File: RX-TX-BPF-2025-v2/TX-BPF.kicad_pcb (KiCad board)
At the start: 11 copper layers, 60.6 x 26.8 mm, 21 parts

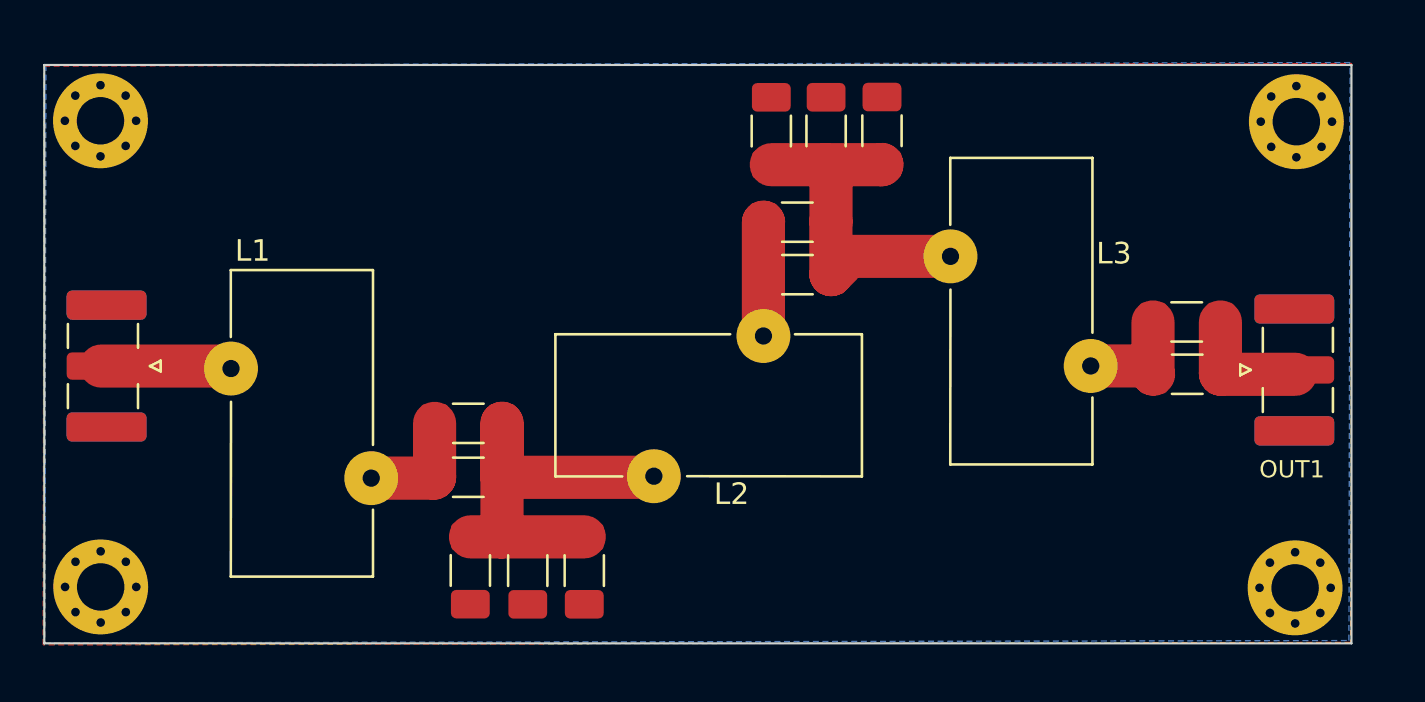
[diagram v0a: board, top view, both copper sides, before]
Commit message: A new start...
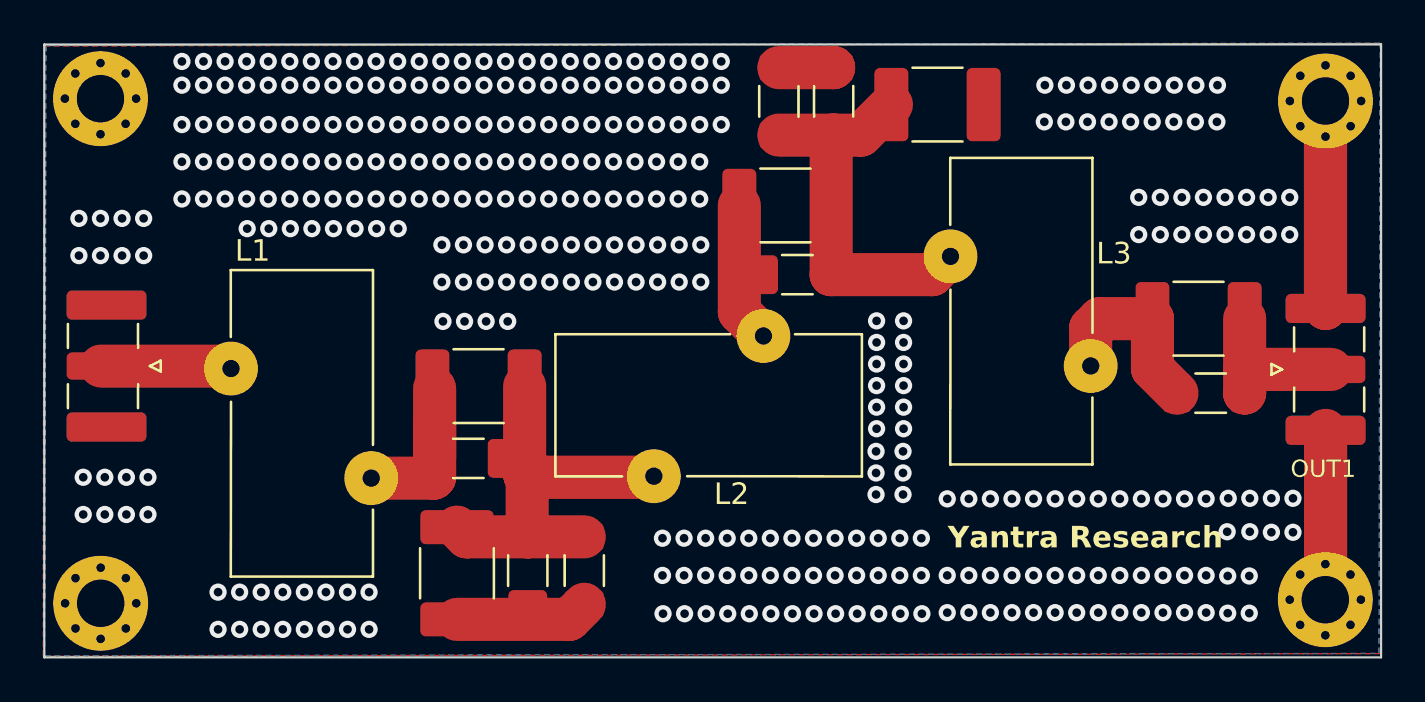
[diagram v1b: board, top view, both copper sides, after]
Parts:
- CFL3, CFS2, CSL2, CSS1, CTS2: footprint Capacitor_SMD:C_1206_3216Metric_Pad1.33x1.80mm_HandSolder -> Capacitor_SMD:C_1812_4532Metric_Pad1.57x3.40mm_HandSolder
- moved CSL2 2.85 mm to (126.8, 85.7), turned to 0 degrees
- moved CFS2 1.79 mm to (105.5, 98.8)
- moved H2 1.66 mm to (144.7, 85.6)
- moved H3 1.50 mm to (144.7, 108.7)
- moved OUT1 1.45 mm to (145.0, 98.0)
- moved CSL3 1.42 mm to (121.9, 85.6)
- moved CSL1 1.42 mm to (119.4, 85.6)
- moved CTS1 1.40 mm to (139.4, 99.1)
- moved H1 1.02 mm to (88.0, 85.5)
- moved CSS1 0.95 mm to (119.7, 90.4)
- moved CFS1 0.88 mm to (105.0, 102.1)
- moved H4 0.76 mm to (88.0, 108.8)
- moved CFL3 0.63 mm to (104.5, 107.5)
- moved CTS2 0.57 mm to (138.8, 95.7)
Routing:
- net GND: track 0.00 -> 26.2 mm, vias 0 -> 340
- net Net-(CTS1-Pad1): track 5.47 -> 8.72 mm
- net Net-(CFS1-Pad2): track 5.45 -> 8.70 mm
- net Net-(CSL1-Pad1): track 16.1 -> 18.2 mm
- net Net-(OUT1-In): track 5.89 -> 7.46 mm
- net Net-(CSS1-Pad1): track 5.28 -> 6.51 mm
- net Net-(CFL1-Pad1): track 20.0 -> 19.0 mm
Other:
- board size 60.6 x 26.8 mm -> 62 x 28.4 mm
- board text added: "Yantra Research"
